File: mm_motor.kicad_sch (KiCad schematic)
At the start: 1 part, among them M1 N20_encoder

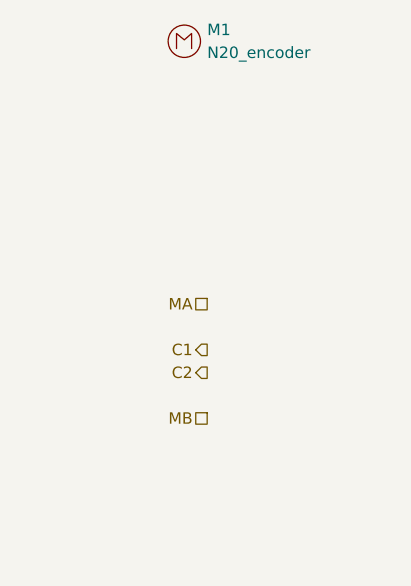
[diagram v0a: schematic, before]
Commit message: tp2
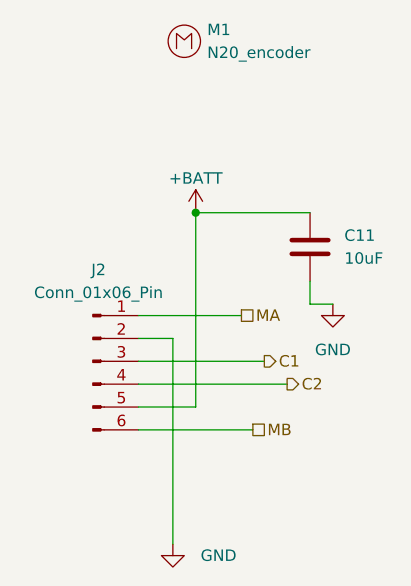
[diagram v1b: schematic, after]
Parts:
- added C11: 10uF, Capacitor_SMD:C_0603_1608Metric, symbol Device:C
- added J2: Conn_01x06_Pin, Connector_PinSocket_2.54mm:PinSocket_1x06_P2.54mm_Vertical, symbol Connector:Conn_01x06_Pin
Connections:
- net C1: now also J2.3 (Pin_3)
- net C2: now also J2.4 (Pin_4)
- net MA: now also J2.1 (Pin_1)
- net MB: now also J2.6 (Pin_6)
- new net +BATT: C11.2, J2.5 (Pin_5)
- new net GND: C11.1, J2.2 (Pin_2)
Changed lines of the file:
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@@
 (kicad_sch (version 20230121) (generator eeschema)
   (paper "A4")
-  (hierarchical_label "C1" (shape output) (at 118.11 91.44 180) (fields_autoplaced)
-    (effects (font (size 1.27 1.27)) (justify right))
-  )
-  (hierarchical_label "C2" (shape output) (at 118.11 93.98 180) (fields_autoplaced)
-    (effects (font (size 1.27 1.27)) (justify right))
-  )
-  (hierarchical_label "MB" (shape passive) (at 118.11 99.06 180) (fields_autoplaced)
-    (effects (font (size 1.27 1.27)) (justify right))
-  )
-  (hierarchical_label "MA" (shape passive) (at 118.11 86.36 180) (fields_autoplaced)
-    (effects (font (size 1.27 1.27)) (justify right))
+  (junction (at 116.84 76.2) (diameter 0) (color 0 0 0 0)
+  )
+  (wire (pts (xy 110.49 100.33) (xy 123.19 100.33))
+    (stroke (width 0) (type default))
+  )
+  (wire (pts (xy 132.08 86.36) (xy 129.54 86.36))
+    (stroke (width 0) (type default))
+  )
+  (wire (pts (xy 129.54 76.2) (xy 116.84 76.2))
+    (stroke (width 0) (type default))
+  )
+  (wire (pts (xy 116.84 76.2) (xy 116.84 97.79))
+    (stroke (width 0) (type default))
+  )
+  (wire (pts (xy 110.49 87.63) (xy 121.92 87.63))
+    (stroke (width 0) (type default))
+  )
+  (wire (pts (xy 129.54 86.36) (xy 129.54 83.82))
+    (stroke (width 0) (type default))
+  )
+  (wire (pts (xy 114.3 90.17) (xy 110.49 90.17))
+    (stroke (width 0) (type default))
+  )
+  (wire (pts (xy 110.49 95.25) (xy 127 95.25))
+    (stroke (width 0) (type default))
+  )
+  (wire (pts (xy 116.84 97.79) (xy 110.49 97.79))
+    (stroke (width 0) (type default))
+  )
+  (wire (pts (xy 110.49 92.71) (xy 124.46 92.71))
+    (stroke (width 0) (type default))
+  )
+  (wire (pts (xy 114.3 113.03) (xy 114.3 90.17))
+    (stroke (width 0) (type default))
+  )
+  (hierarchical_label "C1" (shape output) (at 124.46 92.71 0) (fields_autoplaced)
+    (effects (font (size 1.27 1.27)) (justify left))
+  )
+  (hierarchical_label "C2" (shape output) (at 127 95.25 0) (fields_autoplaced)
+    (effects (font (size 1.27 1.27)) (justify left))
+  )
+  (hierarchical_label "MB" (shape passive) (at 123.19 100.33 0) (fields_autoplaced)
+    (effects (font (size 1.27 1.27)) (justify left))
+  )
+  (hierarchical_label "MA" (shape passive) (at 121.92 87.63 0) (fields_autoplaced)
+    (effects (font (size 1.27 1.27)) (justify left))
+  )
+  (symbol (lib_id "power:GND") (at 132.08 86.36 0) (unit 1)
+    (in_bom yes) (on_board yes) (dnp no) (fields_autoplaced)
+    (property "Reference" "#PWR040" (at 132.08 92.71 0)
+      (effects (font (size 1.27 1.27)) hide)
+    )
+    (property "Value" "GND" (at 132.08 91.44 0)
+      (effects (font (size 1.27 1.27)))
+    )
+    (property "Footprint" "" (at 132.08 86.36 0)
+      (effects (font (size 1.27 1.27)) hide)
+    )
+    (property "Datasheet" "" (at 132.08 86.36 0)
+      (effects (font (size 1.27 1.27)) hide)
+    )
+    (pin "1")
+    (instances
+      (project "minimouse"
+        (path "/d8fa4cba-2469-4231-847f-065b6b829f44/224298a9-7d6e-4a70-a0a5-f2614895ec28"
+          (reference "#PWR040") (unit 1)
+        )
+        (path "/d8fa4cba-2469-4231-847f-065b6b829f44/7f113667-692a-4f4d-b16f-621d32f3f136"
+          (reference "#PWR041") (unit 1)
+        )
+        (path "/d8fa4cba-2469-4231-847f-065b6b829f44/3975acd0-18ad-47bc-9ce1-d8c4d864aafe"
+          (reference "#PWR042") (unit 1)
+        )
+      )
+    )
+  )
+  (symbol (lib_id "power:GND") (at 114.3 113.03 0) (unit 1)
+    (in_bom yes) (on_board yes) (dnp no)
+    (property "Reference" "#PWR027" (at 114.3 119.38 0)
+      (effects (font (size 1.27 1.27)) hide)
+    )
+    (property "Value" "GND" (at 119.38 114.3 0)
+      (effects (font (size 1.27 1.27)))
+    )
+    (property "Footprint" "" (at 114.3 113.03 0)
+      (effects (font (size 1.27 1.27)) hide)
+    )
+    (property "Datasheet" "" (at 114.3 113.03 0)
+      (effects (font (size 1.27 1.27)) hide)
+    )
+    (pin "1")
+    (instances
+      (project "minimouse"
+        (path "/d8fa4cba-2469-4231-847f-065b6b829f44/7f113667-692a-4f4d-b16f-621d32f3f136"
+          (reference "#PWR027") (unit 1)
+        )
+        (path "/d8fa4cba-2469-4231-847f-065b6b829f44/3975acd0-18ad-47bc-9ce1-d8c4d864aafe"
+          (reference "#PWR028") (unit 1)
+        )
+      )
+    )
   )
   (symbol (lib_id "minimouse:N20_w_encoder") (at 115.57 57.15 0) (unit 1)
@@
         )
       )
+    )
+  )
+  (symbol (lib_id "Device:C") (at 129.54 80.01 180) (unit 1)
+    (in_bom yes) (on_board yes) (dnp no) (fields_autoplaced)
+    (property "Reference" "C11" (at 133.35 78.74 0)
+      (effects (font (size 1.27 1.27)) (justify right))
+    )
+    (property "Value" "10uF" (at 133.35 81.28 0)
+      (effects (font (size 1.27 1.27)) (justify right))
+    )
+    (property "Footprint" "Capacitor_SMD:C_0603_1608Metric" (at 128.5748 76.2 0)
+      (effects (font (size 1.27 1.27)) hide)
+    )
+    (property "Datasheet" "~" (at 129.54 80.01 0)
+      (effects (font (size 1.27 1.27)) hide)
+    )
+    (pin "1")
+    (pin "2")
+    (instances
+      (project "minimouse"
+        (path "/d8fa4cba-2469-4231-847f-065b6b829f44/d17bb1c7-f68a-465e-9a17-5858ef86fc30"
+          (reference "C11") (unit 1)
+        )
+        (path "/d8fa4cba-2469-4231-847f-065b6b829f44/7f113667-692a-4f4d-b16f-621d32f3f136"
+          (reference "C13") (unit 1)
+        )
+        (path "/d8fa4cba-2469-4231-847f-065b6b829f44/3975acd0-18ad-47bc-9ce1-d8c4d864aafe"
+          (reference "C14") (unit 1)
+        )
+      )
+    )
+  )
+  (symbol (lib_id "power:+BATT") (at 116.84 76.2 0) (unit 1)
+    (in_bom yes) (on_board yes) (dnp no)
+    (property "Reference" "#PWR030" (at 116.84 80.01 0)
+      (effects (font (size 1.27 1.27)) hide)
+    )
+    (property "Value" "+BATT" (at 116.84 72.39 0)
+      (effects (font (size 1.27 1.27)))
+    )
+    (property "Footprint" "" (at 116.84 76.2 0)
+      (effects (font (size 1.27 1.27)) hide)
+    )
+    (property "Datasheet" "" (at 116.84 76.2 0)
+      (effects (font (size 1.27 1.27)) hide)
+    )
+    (pin "1")
+    (instances
+      (project "minimouse"
+        (path "/d8fa4cba-2469-4231-847f-065b6b829f44/3975acd0-18ad-47bc-9ce1-d8c4d864aafe"
+          (reference "#PWR030") (unit 1)
+        )
+        (path "/d8fa4cba-2469-4231-847f-065b6b829f44/7f113667-692a-4f4d-b16f-621d32f3f136"
+          (reference "#PWR029") (unit 1)
+        )
+      )
+    )
+  )
+  (symbol (lib_id "Connector:Conn_01x06_Pin") (at 105.41 92.71 0) (unit 1)
+    (in_bom yes) (on_board yes) (dnp no) (fields_autoplaced)
+    (property "Reference" "J2" (at 106.045 82.55 0)
+      (effects (font (size 1.27 1.27)))
+    )
+    (property "Value" "Conn_01x06_Pin" (at 106.045 85.09 0)
+      (effects (font (size 1.27 1.27)))
+    )
+    (property "Footprint" "Connector_PinSocket_2.54mm:PinSocket_1x06_P2.54mm_Vertical" (at 105.41 92.71 0)
+      (effects (font (size 1.27 1.27)) hide)
+    )
+    (property "Datasheet" "~" (at 105.41 92.71 0)
+      (effects (font (size 1.27 1.27)) hide)
+    )
+    (pin "5")
+    (pin "2")
+    (pin "4")
+    (pin "6")
+    (pin "3")
+    (pin "1")
+    (instances
+      (project "minimouse"
+        (path "/d8fa4cba-2469-4231-847f-065b6b829f44/7f113667-692a-4f4d-b16f-621d32f3f136"
+          (reference "J2") (unit 1)
+        )
+        (path "/d8fa4cba-2469-4231-847f-065b6b829f44/3975acd0-18ad-47bc-9ce1-d8c4d864aafe"
+          (reference "J3") (unit 1)
+        )
+      )
